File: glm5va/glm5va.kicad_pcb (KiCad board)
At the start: 2 copper layers, 21 parts, among them J1 BANK_xx1, J2 JIN, J3 POWER, U1 74HC245, U2 74HC245

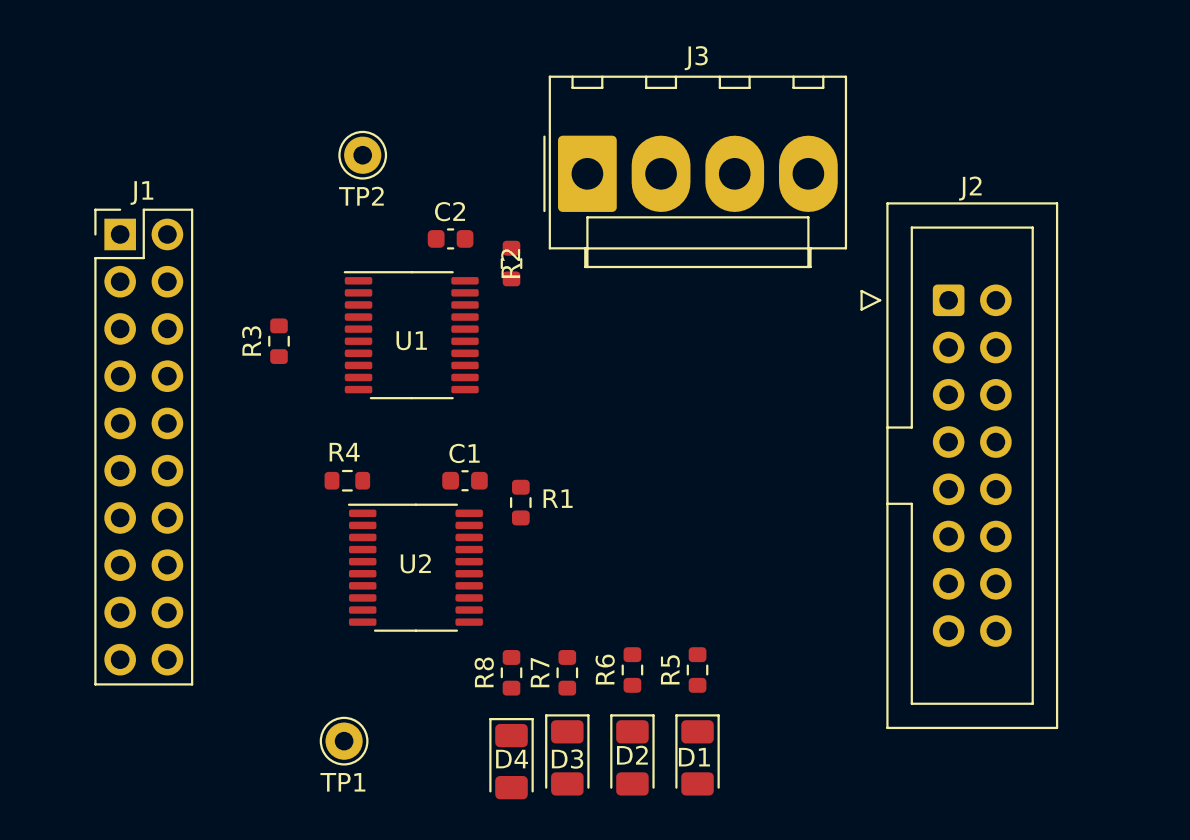
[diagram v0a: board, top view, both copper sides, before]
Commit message: glm5va: routing and layers ok
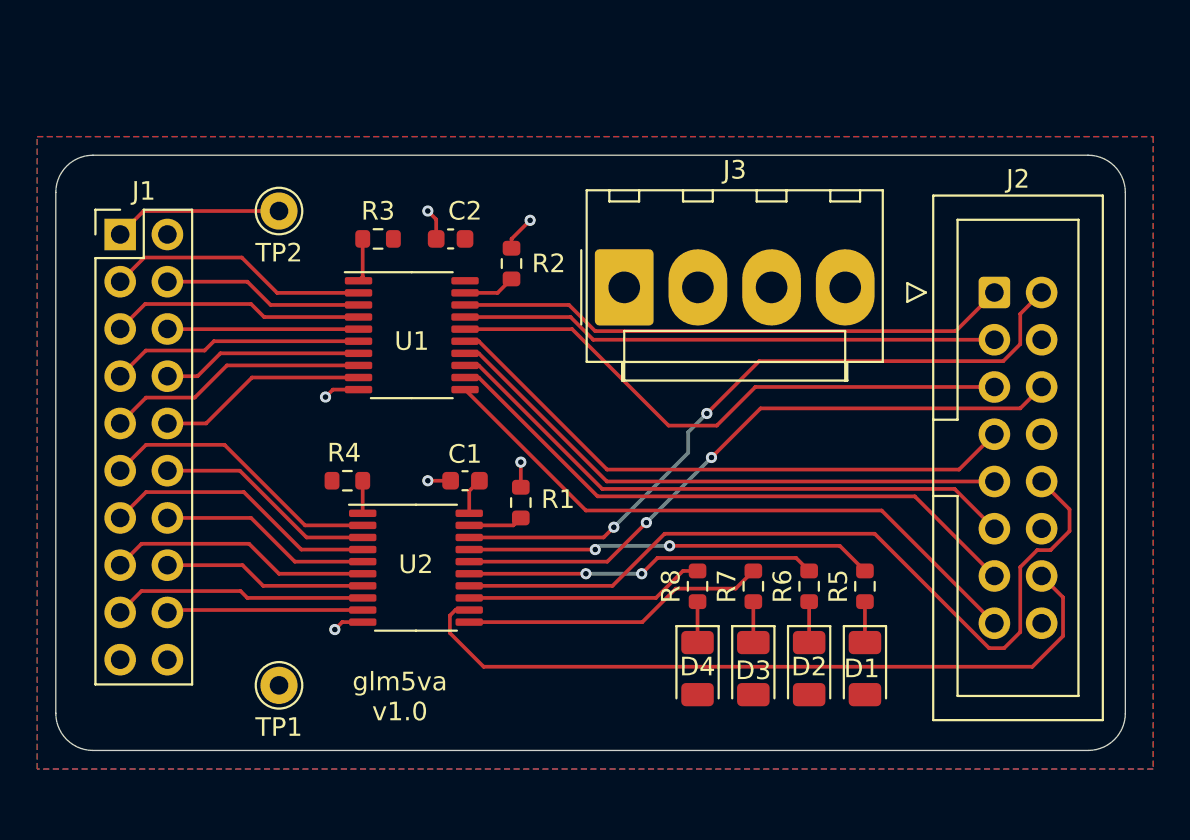
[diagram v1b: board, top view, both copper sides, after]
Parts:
- added G***: LOGO, LOGO, B.Cu at (136.0, 85.0)
- moved D4 11.2 mm to (151.0, 97.1)
- moved D3 11.1 mm to (154.0, 97.1)
- moved R7 11.0 mm to (154.0, 92.7)
- moved R8 11.0 mm to (151.0, 92.7)
- moved D2 10.6 mm to (157.0, 97.1)
- moved R6 10.5 mm to (157.0, 92.7)
- moved D1 10.2 mm to (160.0, 97.1)
- moved R5 10.1 mm to (160.0, 92.7)
- moved R3 7.66 mm to (133.8, 74.0), turned to 180 degrees
- moved J3 6.42 mm to (147.1, 76.6)
- moved TP2 5.41 mm to (128.5, 72.5)
- moved TP1 4.61 mm to (128.5, 98.0)
- moved J2 2.50 mm to (167.0, 76.9)
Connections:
- J1 pad 10: Net-(J1-Pin_10) -> /BANK_B5
- J1 pad 11: Net-(J1-Pin_11) -> /BANK_A4
- J1 pad 12: Net-(J1-Pin_12) -> /BANK_B4
- J1 pad 13: Net-(J1-Pin_13) -> /BANK_A3
- J1 pad 14: Net-(J1-Pin_14) -> /BANK_B3
- J1 pad 15: Net-(J1-Pin_15) -> /BANK_A2
- J1 pad 16: Net-(J1-Pin_16) -> /BANK_B2
- J1 pad 17: Net-(J1-Pin_17) -> /BANK_A1
- J1 pad 18: Net-(J1-Pin_18) -> /BANK_B1
- J1 pad 3: Net-(J1-Pin_3) -> /BANK_A8
- J1 pad 4: Net-(J1-Pin_4) -> /BANK_B8
- J1 pad 5: Net-(J1-Pin_5) -> /BANK_A7
- J1 pad 6: Net-(J1-Pin_6) -> /BANK_B7
- J1 pad 7: Net-(J1-Pin_7) -> /BANK_A6
- J1 pad 8: Net-(J1-Pin_8) -> /BANK_B6
- J1 pad 9: Net-(J1-Pin_9) -> /BANK_A5
- U1 pad 2: Net-(J1-Pin_17) -> /BANK_A8
- U1 pad 3: Net-(J1-Pin_15) -> /BANK_B8
- U1 pad 4: Net-(J1-Pin_13) -> /BANK_A7
- U1 pad 5: Net-(J1-Pin_11) -> /BANK_B7
- U1 pad 6: Net-(J1-Pin_9) -> /BANK_A6
- U1 pad 7: Net-(J1-Pin_7) -> /BANK_B6
- U1 pad 8: Net-(J1-Pin_5) -> /BANK_A5
- U1 pad 9: Net-(J1-Pin_3) -> /BANK_B5
- U2 pad 2: Net-(J1-Pin_18) -> /BANK_A4
- U2 pad 3: Net-(J1-Pin_16) -> /BANK_B4
- U2 pad 4: Net-(J1-Pin_14) -> /BANK_A3
- U2 pad 5: Net-(J1-Pin_12) -> /BANK_B3
- U2 pad 6: Net-(J1-Pin_10) -> /BANK_A2
- U2 pad 7: Net-(J1-Pin_8) -> /BANK_B2
- U2 pad 8: Net-(J1-Pin_6) -> /BANK_A1
- U2 pad 9: Net-(J1-Pin_4) -> /BANK_B1
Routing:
- net /B: track 0.00 -> 43.9 mm
- net /LAT: track 0.00 -> 40.2 mm
- net /G1: track 0.00 -> 37.8 mm, vias 0 -> 2
- net /G2: track 0.00 -> 34.7 mm, vias 0 -> 2
- net /OE: track 0.00 -> 33.7 mm
- net /CLK: track 0.00 -> 32.9 mm
- net /B2: track 0.00 -> 32.1 mm
- net /C: track 0.00 -> 32.1 mm
- net /R2: track 0.00 -> 31.5 mm
- net /A: track 0.00 -> 31.3 mm
- net /R1: track 0.00 -> 29.9 mm
- net /B1: track 0.00 -> 29.0 mm
- net Net-(U2-B1): track 0.00 -> 21.9 mm, vias 0 -> 2
- net Net-(U2-B3): track 0.00 -> 18.9 mm, vias 0 -> 2
- net Net-(U2-B7): track 0.00 -> 16.4 mm
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- added copper zone on F.Cu, net +5V
- added copper zone on B.Cu, net GND
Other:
- board outline added: 57.5 x 32 mm
- board text added: "glm5va v1.0"
